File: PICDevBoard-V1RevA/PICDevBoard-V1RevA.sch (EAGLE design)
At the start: 17 parts, among them IC1 PIC18F2550, J1 DCJ0202

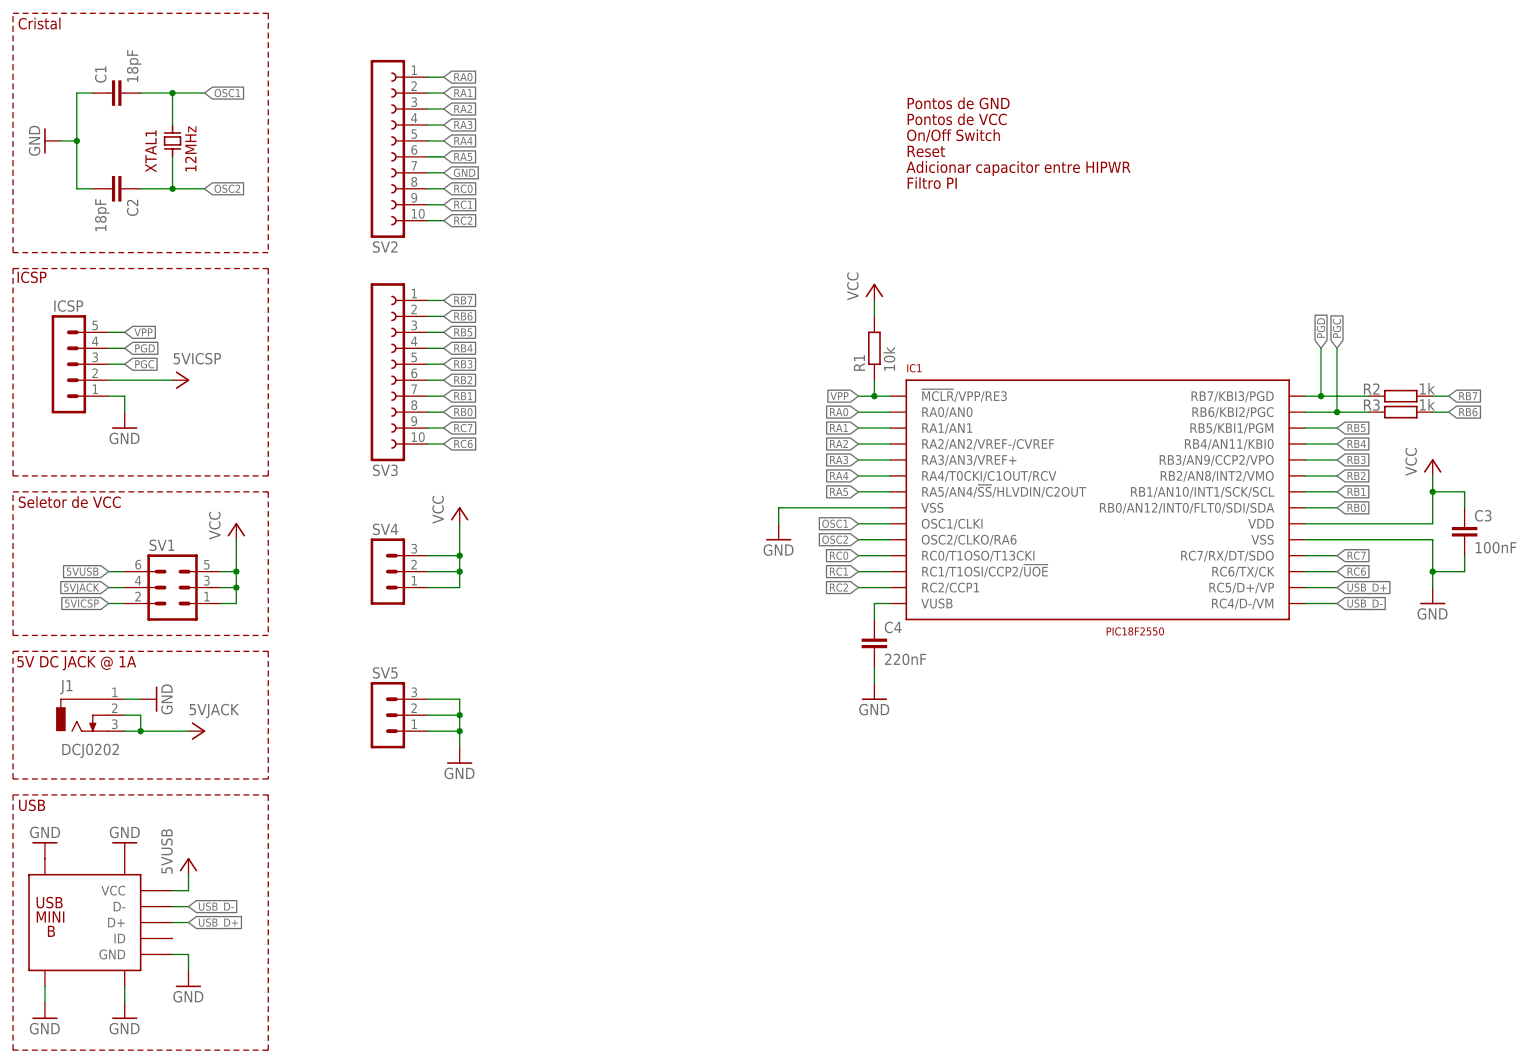
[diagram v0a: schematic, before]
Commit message: Routing
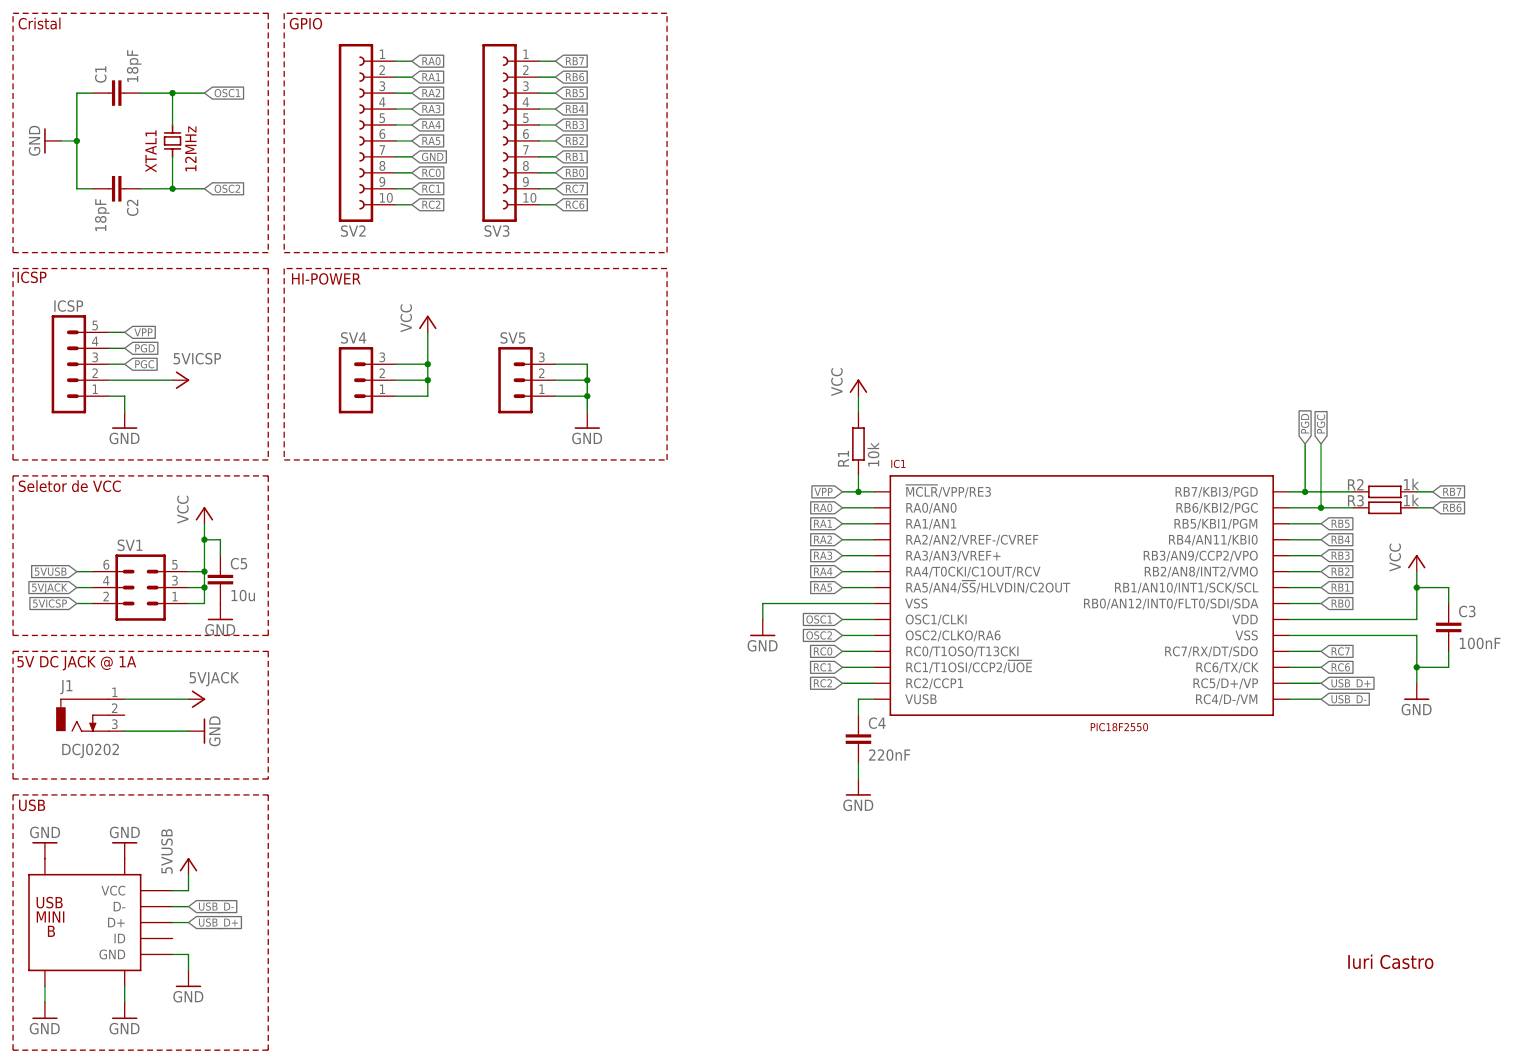
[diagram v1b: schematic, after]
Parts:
- added C5: 10u, rcl:C-EUC0805
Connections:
- net 5VJACK: now also J1.1; no longer J1.2, J1.3
- net GND: now also C5.2, J1.3; no longer J1.1
- net VCC: now also C5.1
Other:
- note added: "GPIO"
- note added: "HI-POWER"
- note added: "Iuri Castro"
- note removed: "Adicionar capacitor entre HIPWR"
- note removed: "Filtro PI"
- note removed: "On/Off Switch"
- note removed: "Pontos de GND"
- note removed: "Pontos de VCC"
- note removed: "Reset"
- moved on the sheet: C3, C4, IC1, R1, R2, R3, SV1, SV2, SV3, SV4, SV5
